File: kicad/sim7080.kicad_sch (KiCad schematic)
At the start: 23 parts, among them J2 USB_C_SIM, J3 SIM_Card, U2 SIM7080G, U6 TXU0204PWR, U7 USBLC6-2SC6

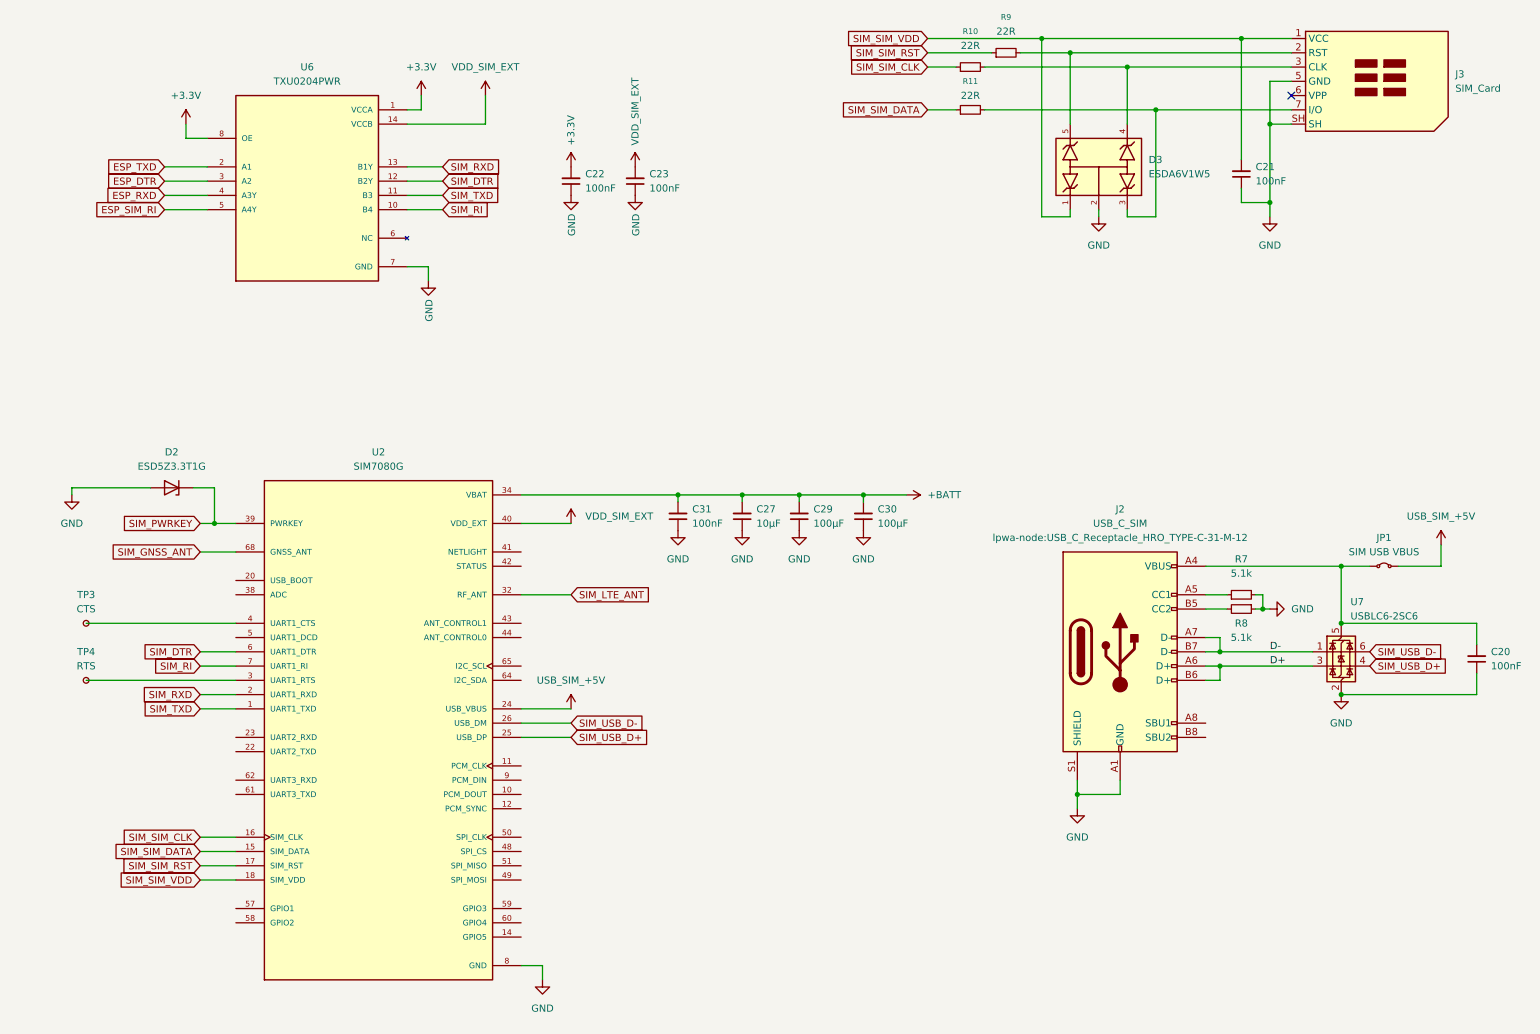
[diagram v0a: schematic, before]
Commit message: Draft
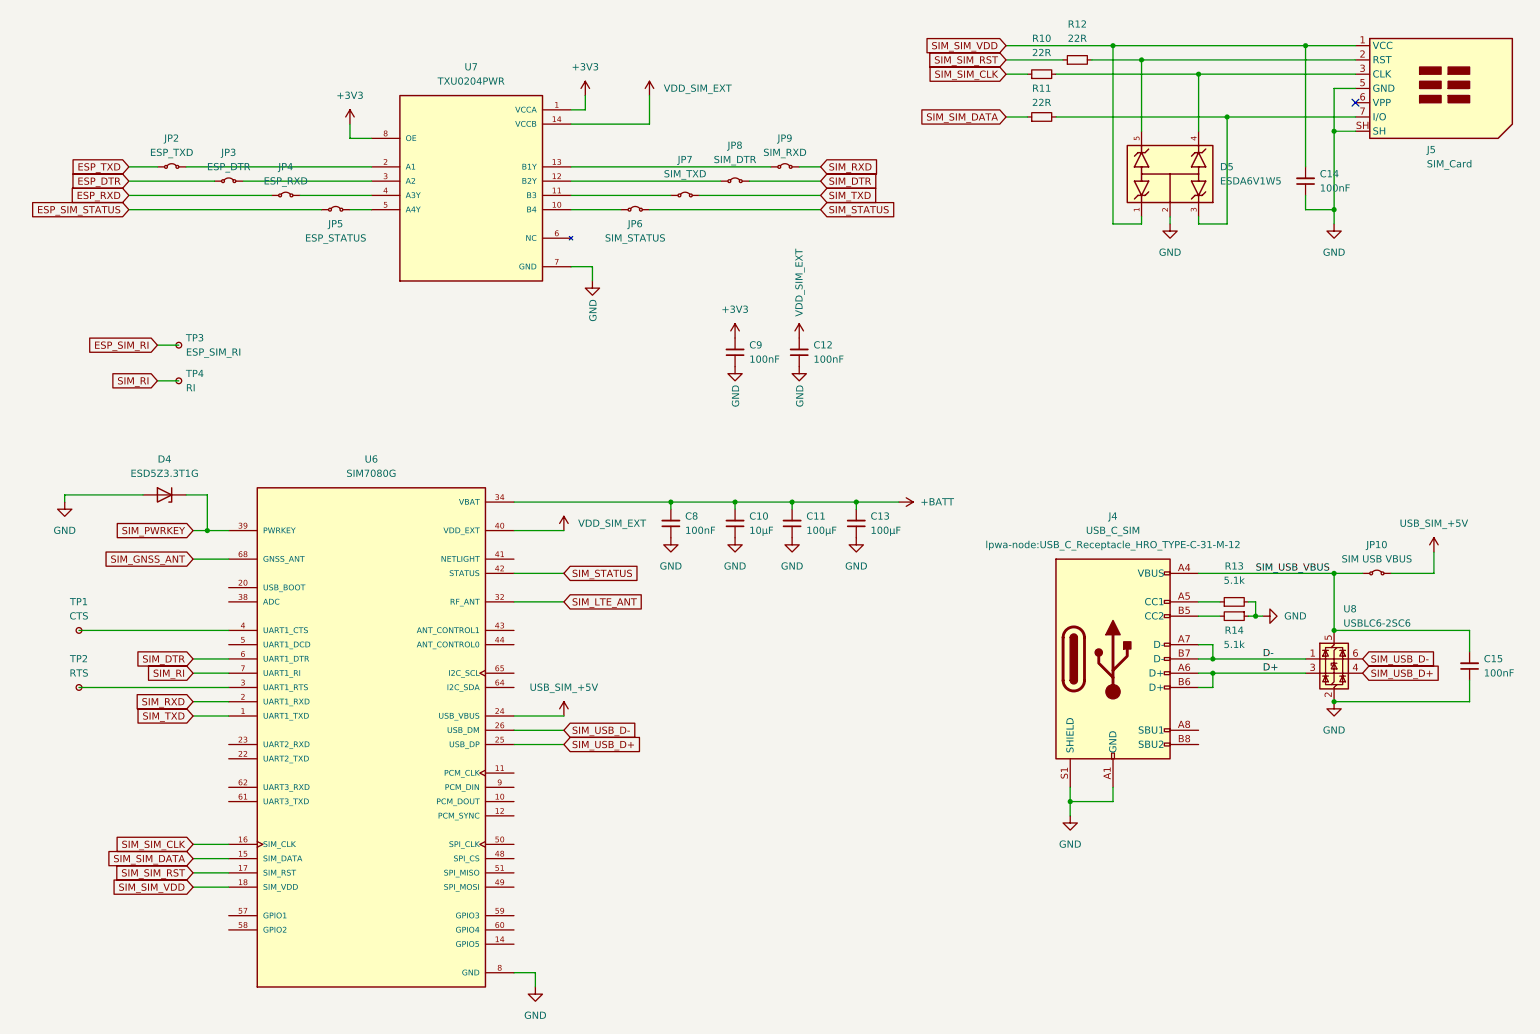
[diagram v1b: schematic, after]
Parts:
- removed C20, C21, C22, C23, C31: 100nF, Capacitor_SMD:C_0603_1608Metric, symbol Device:C_Small
- removed C27: 10µF, Capacitor_SMD:C_0603_1608Metric, symbol Device:C_Small
- removed C29, C30: 100µF, Capacitor_SMD:C_1206_3216Metric, symbol Device:C_Small
- removed D2: ESD5Z3.3T1G, Diode_SMD:D_SOD-523, symbol Diode:ESD5Zxx
- removed D3: ESDA6V1W5, lpwa-node:SOT65P210X110-5N, symbol lpwa-node:ESDA6V1W5
- removed J2: USB_C_SIM, lpwa-node:USB_C_Receptacle_HRO_TYPE-C-31-M-12, symbol Connector:USB_C_Receptacle_USB2.0
- removed J3: SIM_Card, lpwa-node:SMN-304, symbol Connector:SIM_Card_Shielded
- removed JP1: SIM USB VBUS, symbol Jumper:Jumper_2_Small_Bridged
- removed R7, R8: 5.1k, Resistor_SMD:R_0603_1608Metric, symbol Device:R_Small
- removed R9: 22R, symbol Device:R_Small
- removed U2: SIM7080G, lpwa-node:SIM7080G, symbol lpwa-node:SIM7080G
- removed U6: TXU0204PWR, lpwa-node:SOP65P640X120-14N, symbol lpwa-node:TXU0204PWR
- removed U7: USBLC6-2SC6, Package_TO_SOT_SMD:SOT-23-6, symbol Power_Protection:USBLC6-2SC6
- added C10: 10µF, Capacitor_SMD:C_0603_1608Metric, symbol Device:C_Small
- added C11, C13: 100µF, Capacitor_SMD:C_1206_3216Metric, symbol Device:C_Small
- added C12, C14, C15, C8, C9: 100nF, Capacitor_SMD:C_0603_1608Metric, symbol Device:C_Small
- added D4: ESD5Z3.3T1G, Diode_SMD:D_SOD-523, symbol Diode:ESD5Zxx
- added D5: ESDA6V1W5, lpwa-node:SOT65P210X110-5N, symbol lpwa-node:ESDA6V1W5
- added J4: USB_C_SIM, lpwa-node:USB_C_Receptacle_HRO_TYPE-C-31-M-12, symbol Connector:USB_C_Receptacle_USB2.0
- added J5: SIM_Card, lpwa-node:SMN-304, symbol Connector:SIM_Card_Shielded
- added JP10: SIM USB VBUS, lpwa-node:SolderJumper-2_P1.3mm_Bridged_RoundedPad1.0x1.5mm, symbol Jumper:Jumper_2_Small_Bridged
- added JP2: ESP_TXD, lpwa-node:SolderJumper-2_P1.3mm_Bridged_RoundedPad1.0x1.5mm, symbol Jumper:Jumper_2_Small_Bridged
- added JP3: ESP_DTR, lpwa-node:SolderJumper-2_P1.3mm_Bridged_RoundedPad1.0x1.5mm, symbol Jumper:Jumper_2_Small_Bridged
- added JP4: ESP_RXD, lpwa-node:SolderJumper-2_P1.3mm_Bridged_RoundedPad1.0x1.5mm, symbol Jumper:Jumper_2_Small_Bridged
- added JP5: ESP_STATUS, lpwa-node:SolderJumper-2_P1.3mm_Bridged_RoundedPad1.0x1.5mm, symbol Jumper:Jumper_2_Small_Bridged
- added JP6: SIM_STATUS, lpwa-node:SolderJumper-2_P1.3mm_Bridged_RoundedPad1.0x1.5mm, symbol Jumper:Jumper_2_Small_Bridged
- added JP7: SIM_TXD, lpwa-node:SolderJumper-2_P1.3mm_Bridged_RoundedPad1.0x1.5mm, symbol Jumper:Jumper_2_Small_Bridged
- added JP8: SIM_DTR, lpwa-node:SolderJumper-2_P1.3mm_Bridged_RoundedPad1.0x1.5mm, symbol Jumper:Jumper_2_Small_Bridged
- added JP9: SIM_RXD, lpwa-node:SolderJumper-2_P1.3mm_Bridged_RoundedPad1.0x1.5mm, symbol Jumper:Jumper_2_Small_Bridged
- added R12: 22R, Resistor_SMD:R_0603_1608Metric, symbol Device:R_Small
- added R13, R14: 5.1k, Resistor_SMD:R_0603_1608Metric, symbol Device:R_Small
- added TP1: CTS, TestPoint:TestPoint_Pad_D1.5mm, symbol Connector:TestPoint_Small
- added TP2: RTS, TestPoint:TestPoint_Pad_D1.5mm, symbol Connector:TestPoint_Small
- added U6: SIM7080G, lpwa-node:SIM7080G, symbol lpwa-node:SIM7080G
- added U7: TXU0204PWR, lpwa-node:SOP65P640X120-14N, symbol lpwa-node:TXU0204PWR
- added U8: USBLC6-2SC6, Package_TO_SOT_SMD:SOT-23-6, symbol Power_Protection:USBLC6-2SC6
- R10, R11: footprint (none) -> Resistor_SMD:R_0603_1608Metric; LCSC Part # (none) -> C23345
- TP3: value CTS -> ESP_SIM_RI; footprint (none) -> TestPoint:TestPoint_Pad_D1.5mm
- TP4: value RTS -> RI; footprint (none) -> TestPoint:TestPoint_Pad_D1.5mm
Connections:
- net +BATT: now also C10.2, C11.2, C13.2, C8.2, U6.34 (VBAT), U6.35 (VBAT)
- net D+: now also J4.A6 (D+), J4.B6 (D+), U8.3 (I/O2)
- net D-: now also J4.A7 (D-), J4.B7 (D-), U8.1 (I/O1)
- net ESP_DTR: now also JP3.1 (A)
- net ESP_RXD: now also JP4.1 (A)
- net ESP_SIM_RI: now also TP3.1
- net ESP_TXD: now also JP2.1 (A)
- net GND: now also C10.1, C11.1, C12.1, C13.1, C14.1, C15.1, C8.1, C9.1, D4.2 (A), D5.2, J4.A1 (GND), J4.A12 (GND), J4.B1 (GND), J4.B12 (GND), J4.S1 (SHIELD), J5.5 (GND), J5.SH, R13.2, R14.1, U6.13 (GND), U6.19 (GND), U6.21 (GND), U6.27 (GND), U6.30 (GND), U6.31 (GND), U6.33 (GND), U6.36 (GND), U6.37 (GND), U6.45 (GND), U6.63 (GND), U6.66 (GND), U6.67 (GND), U6.69 (GND), U6.70 (GND), U6.71 (GND), U6.72 (GND), U6.73 (GND), U6.74 (GND), U6.75 (GND), U6.76 (GND), U6.77 (GND), U6.8 (GND), U7.7 (GND), U8.2 (GND)
- net SIM_DTR: now also JP8.2 (B), U6.6 (UART1_DTR)
- net SIM_GNSS_ANT: now also U6.68 (GNSS_ANT)
- net SIM_LTE_ANT: now also U6.32 (RF_ANT)
- net SIM_PWRKEY: now also D4.1 (K), U6.39 (PWRKEY)
- net SIM_RI: now also TP4.1, U6.7 (UART1_RI)
- net SIM_RXD: now also JP9.2 (B), U6.2 (UART1_RXD)
- net SIM_SIM_CLK: now also U6.16 (SIM_CLK)
- net SIM_SIM_DATA: now also U6.15 (SIM_DATA)
- net SIM_SIM_RST: now also R12.1, U6.17 (SIM_RST)
- net SIM_SIM_VDD: now also C14.2, D5.1, J5.1 (VCC), U6.18 (SIM_VDD)
- net SIM_TXD: now also JP7.2 (B), U6.1 (UART1_TXD)
- net SIM_USB_D+: now also U6.25 (USB_DP), U8.4 (I/O2)
- net SIM_USB_D-: now also U6.26 (USB_DM), U8.6 (I/O1)
- net USB_SIM_+5V: now also JP10.2 (B), U6.24 (USB_VBUS)
- net VDD_SIM_EXT: now also C12.2, U6.40 (VDD_EXT), U7.14 (VCCB)
- net at R11.2: now also D5.3, J5.7 (I/O)
- net at R10.2: now also D5.4, J5.3 (CLK)
- new net: TP1.1, U6.4 (UART1_CTS)
- new net: TP2.1, U6.3 (UART1_RTS)
- new net: JP9.1 (A), U7.13 (B1Y)
- new net: JP4.2 (B), U7.4 (A3Y)
- new net: JP6.1 (A), U7.10 (B4)
- new net: JP7.1 (A), U7.11 (B3)
- new net: JP8.1 (A), U7.12 (B2Y)
- new net: JP2.2 (B), U7.2 (A1)
- new net: JP3.2 (B), U7.3 (A2)
- new net: JP5.2 (B), U7.5 (A4Y)
- new net: U7.6 (NC), U7.9 (NC)
- new net: J4.B5 (CC2), R14.2
- new net: D5.5, J5.2 (RST), R12.2
- new net: J4.A5 (CC1), R13.1
- new net +3V3: C9.2, U7.1 (VCCA), U7.8 (OE)
- new net ESP_SIM_STATUS: JP5.1 (A)
- new net SIM_STATUS: JP6.2 (B), U6.42 (STATUS)
- new net SIM_USB_VBUS: C15.2, J4.A4 (VBUS), J4.A9 (VBUS), J4.B4 (VBUS), J4.B9 (VBUS), JP10.1 (A), U8.5 (VBUS)
